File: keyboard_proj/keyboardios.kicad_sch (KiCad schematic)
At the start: 23 parts, among them J1 Conn_02x04_Odd_Even, J2 Conn_01x32, U6 XL9555QF24

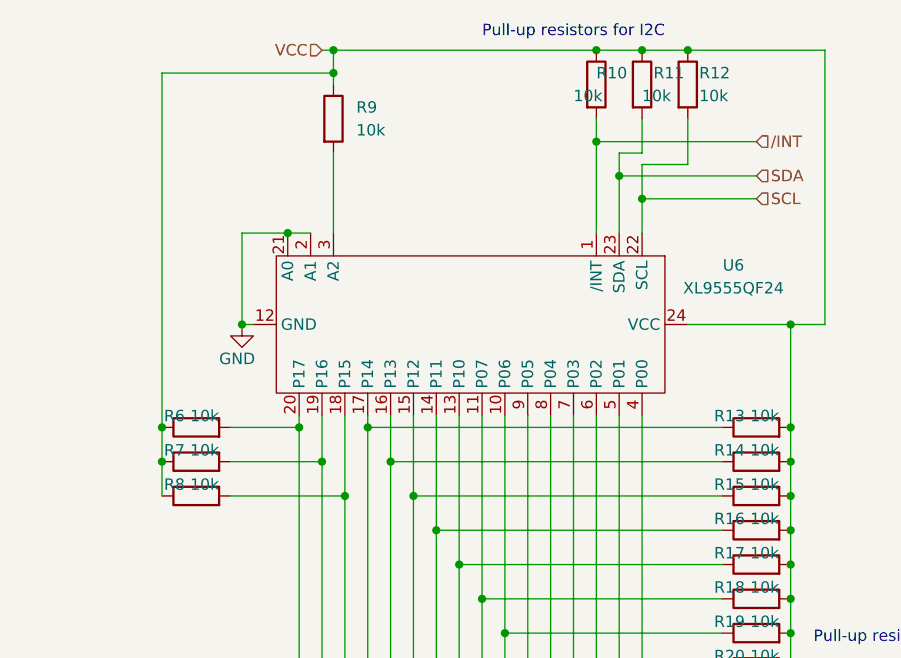
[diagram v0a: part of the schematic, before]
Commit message: PCB bien avancé, presque fini mais je dois selectionner des pieces de jlcpcb pour baisser les couts
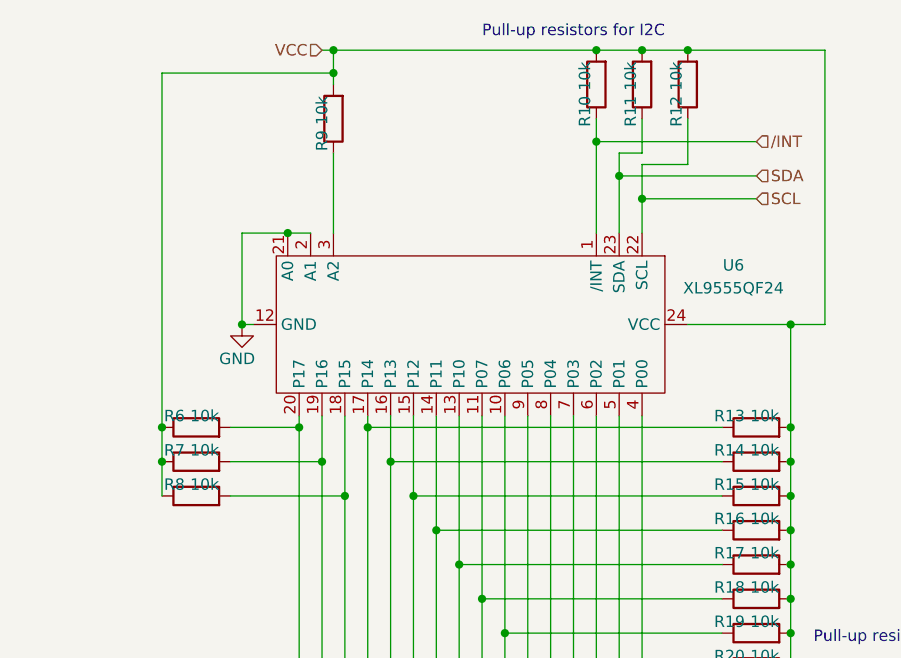
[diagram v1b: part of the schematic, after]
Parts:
- J1: LCSC (none) -> C376087
- J2: LCSC (none) -> C2842545
- R10, R11, R12, R13, R14, R15, R16, R17, R18, R19, R20, R21, R22, R23, R24, R25, R6, R7, R8, R9: LCSC (none) -> C2692697
- U6: LCSC (none) -> C5125492
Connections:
- net SCL: now also R12.1; no longer R12.2
- net SDA: now also R11.1; no longer R11.2
- net VCC: now also R10.2, R11.2, R12.2, R9.2; no longer R10.1, R11.1, R12.1, R9.1
- net /INT: now also R10.1; no longer R10.2
- net at U6.3 (A2): now also R9.1; no longer R9.2
